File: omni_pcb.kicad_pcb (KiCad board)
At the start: 2 copper layers, 116.5 x 85.5 mm, 30 parts

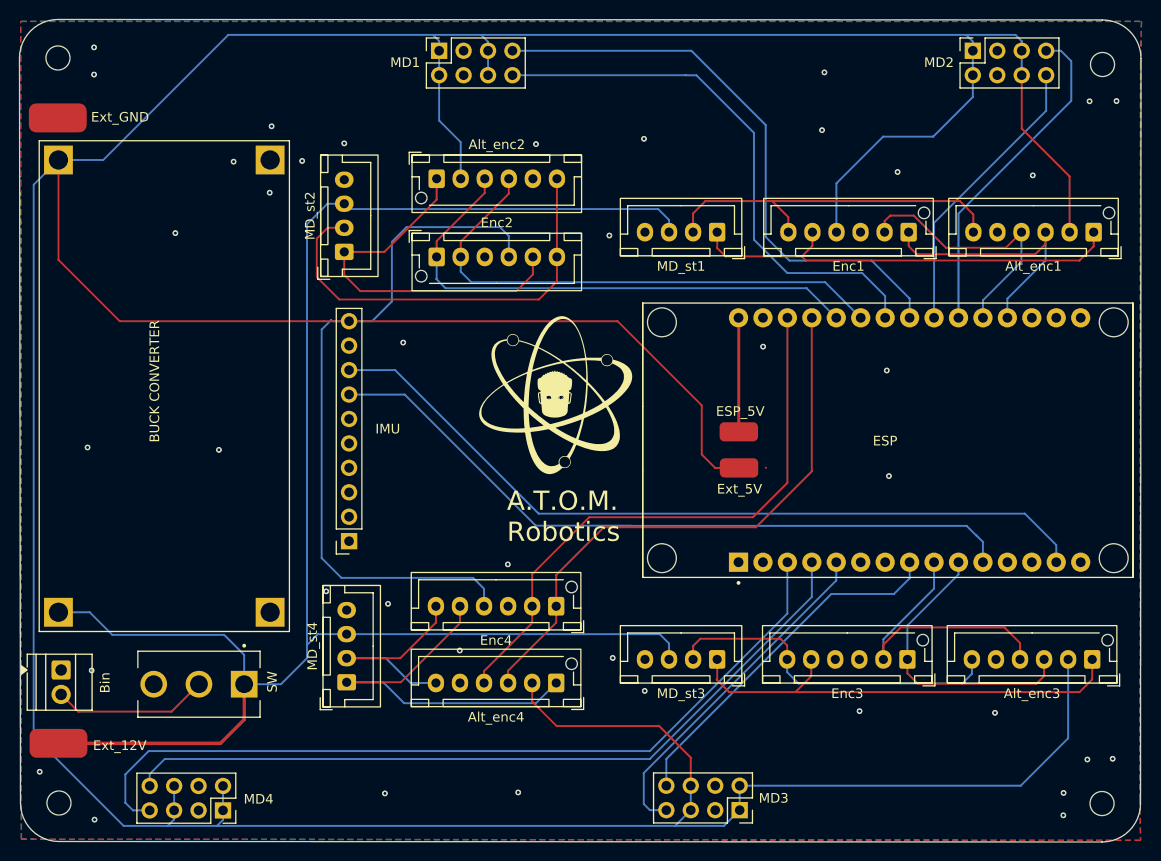
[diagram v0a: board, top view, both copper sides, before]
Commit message: pcb final
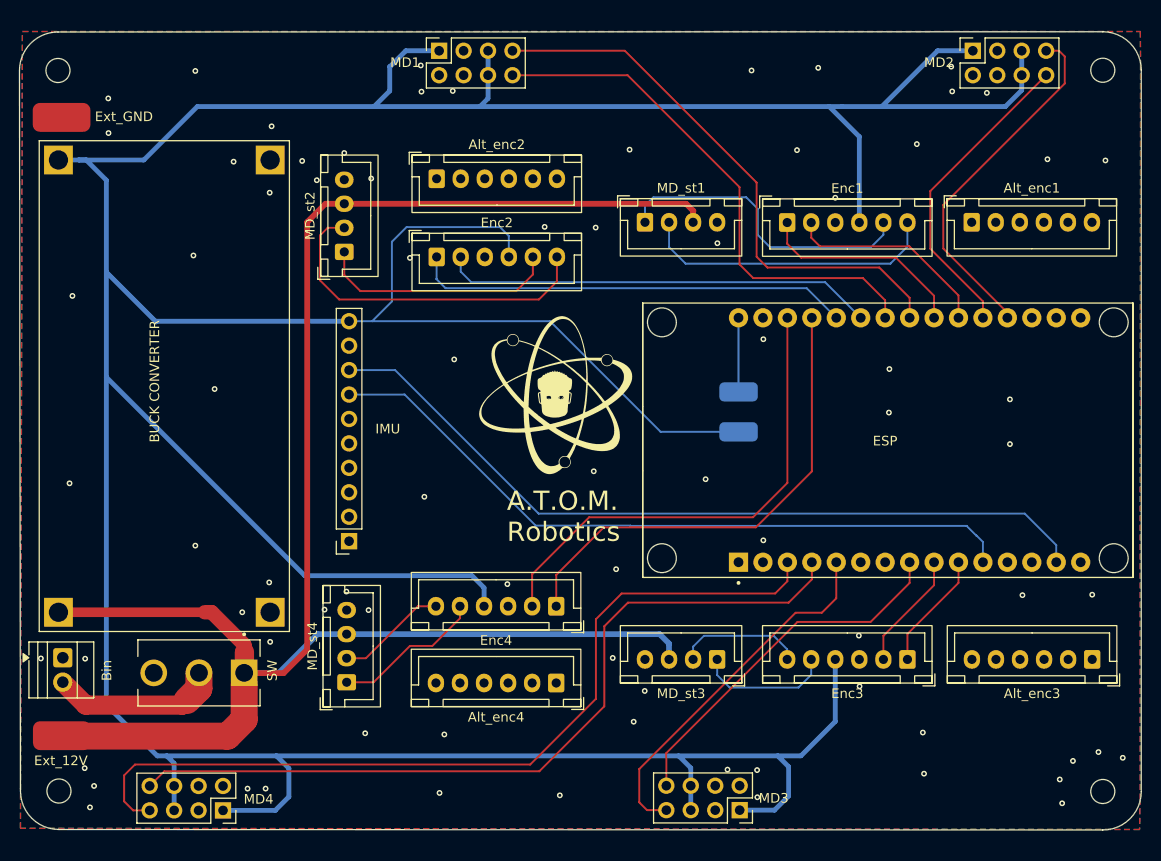
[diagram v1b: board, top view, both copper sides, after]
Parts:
- Alt_enc1, Alt_enc2, Alt_enc3, Alt_enc4, Enc1, Enc2, Enc3, Enc4: footprint Connector_JST:JST_XH_B6B-XH-AM_1x06_P2.50mm_Vertical -> Connector_JST:JST_XH_B6B-XH-A_1x06_P2.50mm_Vertical
- moved Alt_enc1 12.7 mm to (177.9, 40.1), turned to 0 degrees
- moved Enc1 12.7 mm to (158.8, 40.1), turned to 0 degrees
- moved MD_st1 7.57 mm to (144.0, 40.1), turned to 0 degrees
- moved ESP_5V1 4.15 mm to (153.7, 57.7)
- moved Ext_5V1 3.75 mm to (153.7, 61.9)
- moved H4 1.30 mm to (83.0, 24.3)
- moved Bin1 1.29 mm to (83.5, 85.3)
- moved H1 1.25 mm to (191.6, 99.2)
- moved H2 1.25 mm to (83.1, 99.2)
- moved B-SW_1 1.18 mm to (97.7, 86.9)
- moved Ext_12V1 0.87 mm to (83.4, 93.4)
- moved H3 0.60 mm to (191.6, 24.3)
- moved Ext_GND1 0.40 mm to (83.4, 29.2)
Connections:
- Alt_enc1 pad 1: /M+1 -> unconnected-(Alt_enc1-Pin_1-Pad1)
- Alt_enc1 pad 2: +5V -> unconnected-(Alt_enc1-Pin_2-Pad2)
- Alt_enc1 pad 3: /M1_ChB -> unconnected-(Alt_enc1-Pin_3-Pad3)
- Alt_enc1 pad 4: /M1_ChA -> unconnected-(Alt_enc1-Pin_4-Pad4)
- Alt_enc1 pad 5: GND -> unconnected-(Alt_enc1-Pin_5-Pad5)
- Alt_enc1 pad 6: /M-1 -> unconnected-(Alt_enc1-Pin_6-Pad6)
- Alt_enc2 pad 1: /M+2 -> unconnected-(Alt_enc2-Pin_1-Pad1)
- Alt_enc2 pad 2: +5V -> unconnected-(Alt_enc2-Pin_2-Pad2)
- Alt_enc2 pad 3: /M2_ChB -> unconnected-(Alt_enc2-Pin_3-Pad3)
- Alt_enc2 pad 4: /M2_ChA -> unconnected-(Alt_enc2-Pin_4-Pad4)
- Alt_enc2 pad 5: GND -> unconnected-(Alt_enc2-Pin_5-Pad5)
- Alt_enc2 pad 6: /M-2 -> unconnected-(Alt_enc2-Pin_6-Pad6)
- Alt_enc3 pad 1: /M+3 -> unconnected-(Alt_enc3-Pin_1-Pad1)
- Alt_enc3 pad 2: +5V -> unconnected-(Alt_enc3-Pin_2-Pad2)
- Alt_enc3 pad 3: /M3_ChB -> unconnected-(Alt_enc3-Pin_3-Pad3)
- Alt_enc3 pad 4: /M3_ChA -> unconnected-(Alt_enc3-Pin_4-Pad4)
- Alt_enc3 pad 5: GND -> unconnected-(Alt_enc3-Pin_5-Pad5)
- Alt_enc3 pad 6: /M-3 -> unconnected-(Alt_enc3-Pin_6-Pad6)
- Alt_enc4 pad 1: /M+4 -> unconnected-(Alt_enc4-Pin_1-Pad1)
- Alt_enc4 pad 2: +5V -> unconnected-(Alt_enc4-Pin_2-Pad2)
- Alt_enc4 pad 3: /M4_ChB -> unconnected-(Alt_enc4-Pin_3-Pad3)
- Alt_enc4 pad 4: /M4_ChA -> unconnected-(Alt_enc4-Pin_4-Pad4)
- Alt_enc4 pad 5: GND -> unconnected-(Alt_enc4-Pin_5-Pad5)
- Alt_enc4 pad 6: /M-4 -> unconnected-(Alt_enc4-Pin_6-Pad6)
- ESP1 pad 19: /M1_ChB -> /R_PWM_2
- ESP1 pad 20: /M1_ChA -> /L_PWM_2
- ESP1 pad 21: /R_PWM_2 -> /M1_ChA
- ESP1 pad 22: /L_PWM_2 -> /M1_ChB
- MD1 pad 2: +5V -> GND
- MD2 pad 2: +5V -> GND
- MD3 pad 2: +5V -> GND
- MD4 pad 2: +5V -> GND
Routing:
- net +5V: track 568.2 -> 475.2 mm
- net /M+3: track 48.4 -> 14.1 mm
- net /M+4: track 39.6 -> 15.8 mm
- net /M-3: track 36.2 -> 13.2 mm
- net /M3_ChA: track 31.1 -> 12.3 mm
- net /M3_ChB: track 30.5 -> 12.3 mm
- net /M+2: track 39.3 -> 25.2 mm
- net /M+1: track 46.4 -> 32.4 mm
- net /M-4: track 22.8 -> 11.5 mm
- net /M2_ChB: track 55.7 -> 45.5 mm
- net /M2_ChA: track 55.3 -> 45.1 mm
- net /M4_ChB: track 60.3 -> 50.2 mm
- net /M4_ChA: track 61.0 -> 50.9 mm
- net /Vin: track 182.4 -> 191.1 mm
- net /M-2: track 44.7 -> 36.3 mm
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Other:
- board size 116.5 x 85.5 mm -> 116.6 x 82.9 mm
